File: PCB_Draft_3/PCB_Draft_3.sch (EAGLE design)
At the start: 24 parts, among them SW1 PUSHBUTTON, SW2 PUSHBUTTON

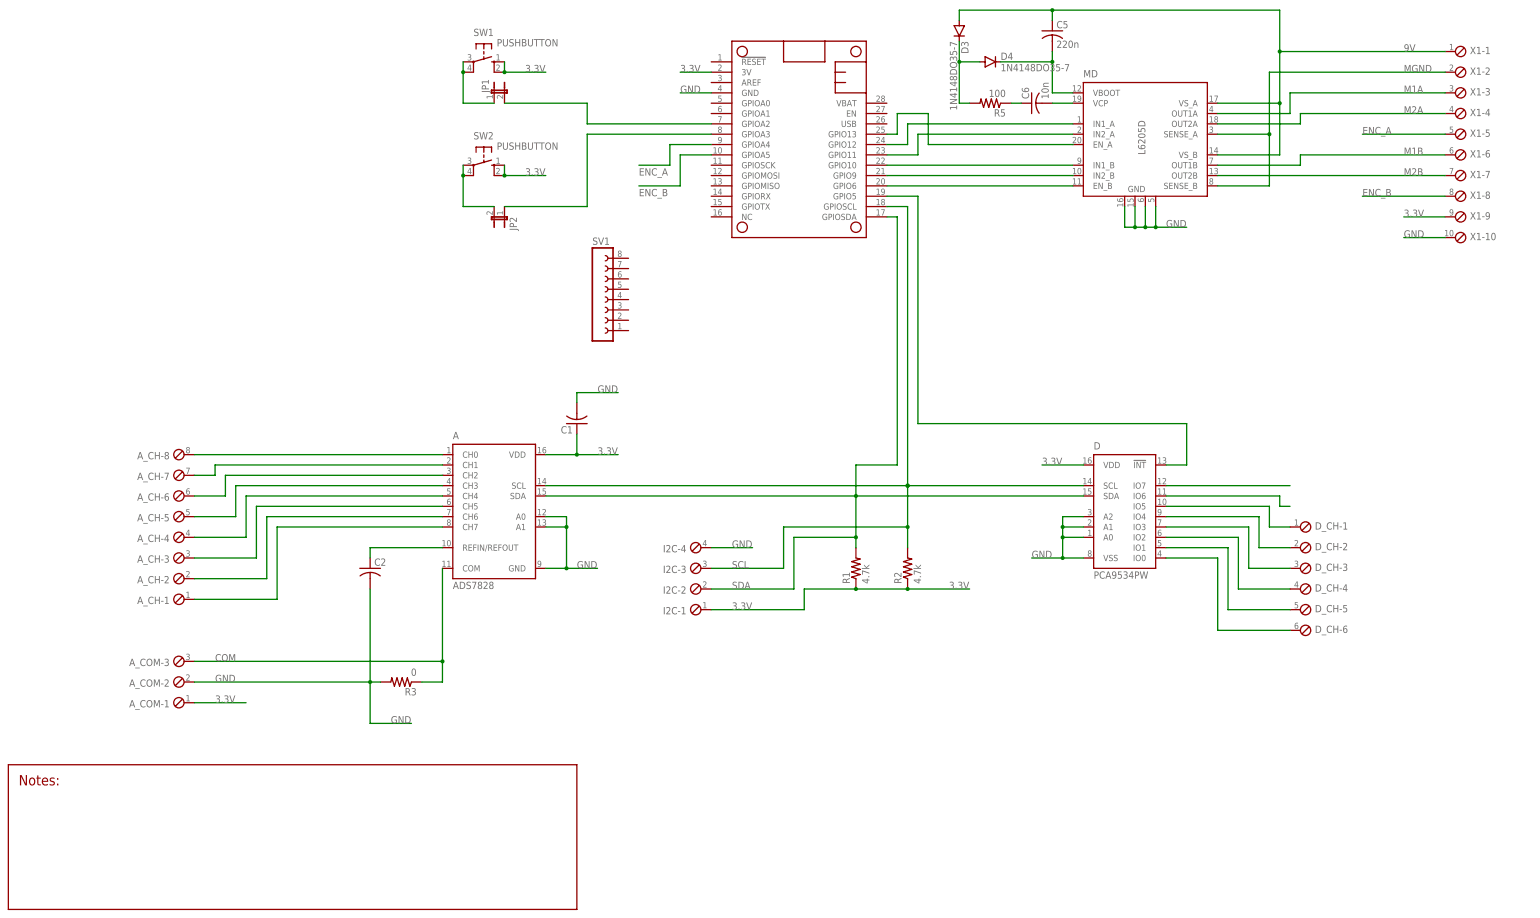
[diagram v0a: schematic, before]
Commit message: Near-final draft - all wires run; checking formatting
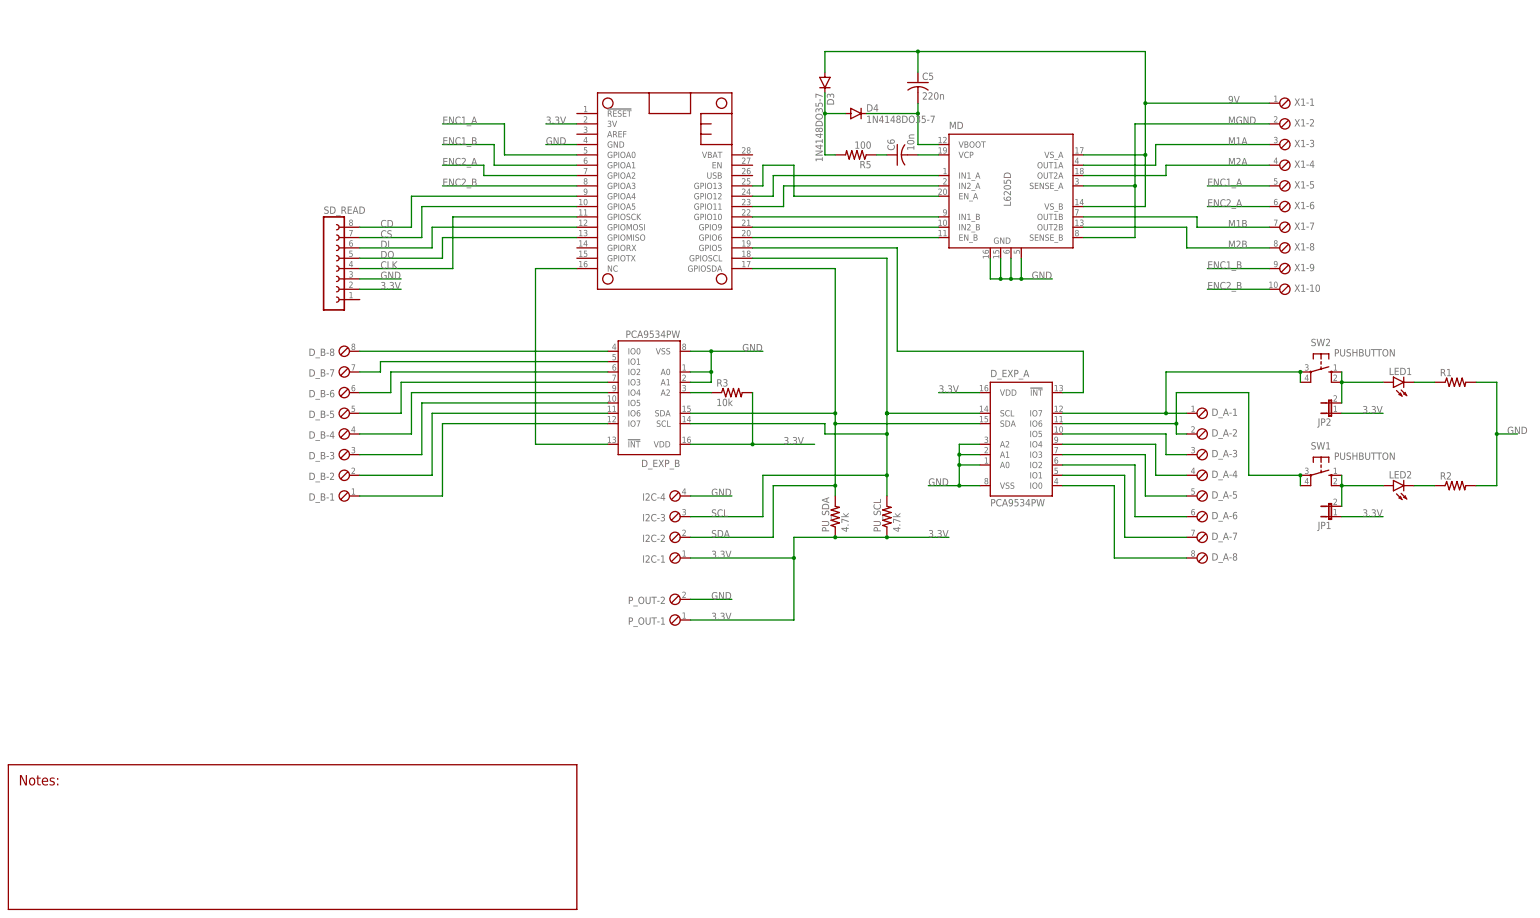
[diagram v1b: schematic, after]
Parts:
- removed A: ADS7828, burr-brown:ADS7828
- removed A_CH: (no value), ME507:SCREWTERM_8P_254
- removed A_COM: (no value), ME507:SCREWTERM_3P_254
- removed C1, C2: (no value), rcl:C-USC0805
- removed D: PCA9534PW, micro-philips:PCA9534PW
- removed D_CH: (no value), ME507:SCREWTERM_6P_254
- removed SV1: (no value), con-lsta:FE08-1
- added D_A, D_B: (no value), ME507:SCREWTERM_8P_254
- added D_EXP_A, D_EXP_B: PCA9534PW, micro-philips:PCA9534PW
- added LED1, LED2: (no value), led:LEDCHIPLED_0805
- added PU_SCL, PU_SDA: 4.7k, rcl:R-US_M0805
- added P_OUT: (no value), ME507:SCREWTERM_2P_254
- added SD_READ: (no value), con-lsta:FE08-1
- R1, R2: value 4.7k -> (none)
- R3: value 0 -> 10k
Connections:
- removed net COM: A.COM, A_COM-3.1, R3.1
- removed net ENC_A: FTHRWNG.GPIOA4, X1-5.1
- removed net ENC_B: FTHRWNG.GPIOA5, X1-8.1
- removed net N$30: FTHRWNG.GPIOA2, JP1.2
- new net CD: FTHRWNG.GPIOA4, SD_READ.8
- new net CLK: FTHRWNG.GPIOSCK, SD_READ.4
- new net CS: FTHRWNG.GPIOA5, SD_READ.7
- new net DI: FTHRWNG.GPIOMOSI, SD_READ.6
- new net DO: FTHRWNG.GPIOMISO, SD_READ.5
- new net ENC1_A: FTHRWNG.GPIOA0, X1-5.1
- new net ENC1_B: FTHRWNG.GPIOA1, X1-9.1
- new net ENC2_A: FTHRWNG.GPIOA2, X1-6.1
- new net ENC2_B: FTHRWNG.GPIOA3, X1-10.1
- new net N$24: JP2.2, LED1.A, SW2.S, SW2.S1
- new net N$28: LED1.C, R1.1
- net 3.3V: now also D_EXP_A.VDD, D_EXP_B.VDD, JP1.1, JP2.1, PU_SCL.1, PU_SDA.1, P_OUT-1.1, R3.2, SD_READ.2; no longer A.VDD, A_COM-1.1, C1.1, D.VDD, R1.1, R2.1, SW1.S, SW1.S1, SW2.S, SW2.S1, X1-9.1
- net GND: now also D_EXP_A.A0, D_EXP_A.A1, D_EXP_A.A2, D_EXP_A.VSS, D_EXP_B.A0, D_EXP_B.A1, D_EXP_B.VSS, P_OUT-2.1, R1.2, R2.2, SD_READ.3; no longer A.A0, A.A1, A.GND, A_COM-2.1, C1.2, C2.2, D.A0, D.A1, D.A2, D.VSS, R3.2, X1-10.1
- net M1B: now also X1-7.1; no longer X1-6.1
- net M2B: now also X1-8.1; no longer X1-7.1
- net N$1: now also D_A-1.1, D_EXP_A.IO7, SW2.P, SW2.P1; no longer D.IO7
- net N$10: now also D_B-7.1, D_EXP_B.IO1; no longer A.CH1, A_CH-7.1
- net N$11: now also D_B-6.1, D_EXP_B.IO2; no longer A.CH2, A_CH-6.1
- net N$12: now also D_B-5.1, D_EXP_B.IO3; no longer A.CH3, A_CH-5.1
- net N$13: now also D_B-4.1, D_EXP_B.IO4; no longer A.CH4, A_CH-4.1
- net N$14: now also D_B-3.1, D_EXP_B.IO5; no longer A.CH5, A_CH-3.1
- net N$15: now also D_B-2.1, D_EXP_B.IO6; no longer A.CH6, A_CH-2.1
- net N$16: now also D_B-1.1, D_EXP_B.IO7; no longer A.CH7, A_CH-1.1
- net N$17: now also LED2.C, R2.1; no longer A.REFIN/REFOUT, C2.1
- net N$19: now also D_EXP_A.!INT; no longer D.!INT
- net N$2: now also D_A-2.1, D_EXP_A.IO6, SW1.P, SW1.P1; no longer D.IO6
- net N$26: now also JP1.2, LED2.A, SW1.S, SW1.S1; no longer JP1.1, SW1.P, SW1.P1
- net N$27: now also D_EXP_B.!INT, FTHRWNG.NC; no longer JP2.2, SW2.P, SW2.P1
- net N$29: now also D_EXP_B.A2, R3.1; no longer FTHRWNG.GPIOA3, JP2.1
- net N$3: now also D_A-3.1, D_EXP_A.IO5; no longer D.IO5, D_CH-1.1
- net N$4: now also D_A-4.1, D_EXP_A.IO4; no longer D.IO4, D_CH-2.1
- net N$5: now also D_A-5.1, D_EXP_A.IO3; no longer D.IO3, D_CH-3.1
- net N$6: now also D_A-6.1, D_EXP_A.IO2; no longer D.IO2, D_CH-4.1
- net N$7: now also D_A-7.1, D_EXP_A.IO1; no longer D.IO1, D_CH-5.1
- net N$8: now also D_A-8.1, D_EXP_A.IO0; no longer D.IO0, D_CH-6.1
- net N$9: now also D_B-8.1, D_EXP_B.IO0; no longer A.CH0, A_CH-8.1
- net SCL: now also D_EXP_A.SCL, D_EXP_B.SCL, PU_SCL.2; no longer A.SCL, D.SCL, R2.2
- net SDA: now also D_EXP_A.SDA, D_EXP_B.SDA, PU_SDA.2; no longer A.SDA, D.SDA, R1.2
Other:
- moved on the sheet: C5, C6, D3, D4, I2C-1, I2C-2, I2C-3, I2C-4, JP1, JP2, MD, R1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
